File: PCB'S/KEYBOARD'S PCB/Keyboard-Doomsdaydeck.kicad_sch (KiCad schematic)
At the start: 2 parts, among them J5 Conn_01x04_Pin, U1 Raspberry_Pi_Pico2

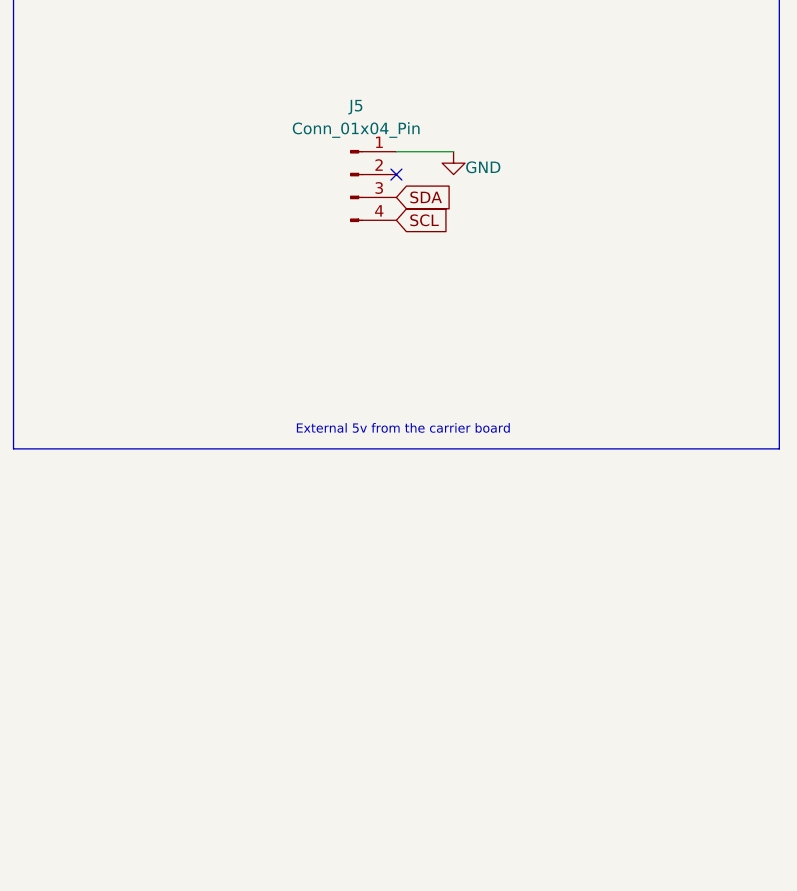
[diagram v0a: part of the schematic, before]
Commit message: ain
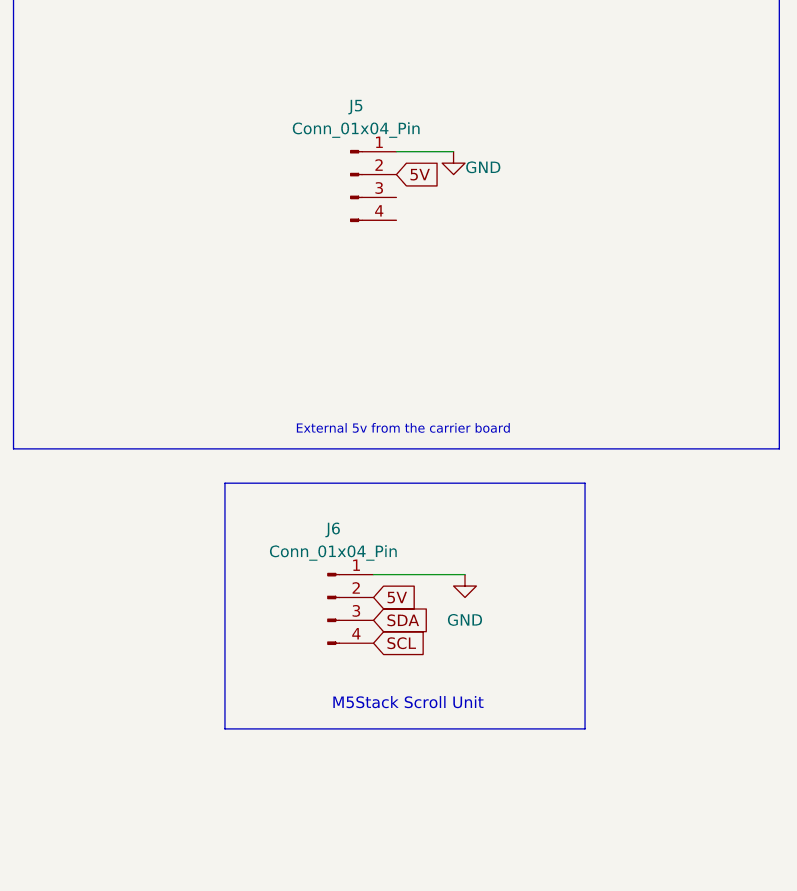
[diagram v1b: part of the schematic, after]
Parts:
- added J6: Conn_01x04_Pin, Connector:FanPinHeader_1x04_P2.54mm_Vertical, symbol Connector:Conn_01x04_Pin
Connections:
- net GND: now also J6.1 (Pin_1)
- net SCL: now also J6.4 (Pin_4); no longer J5.4 (Pin_4)
- net SDA: now also J6.3 (Pin_3); no longer J5.3 (Pin_3)
- net 5V: now reaches J5.2 (Pin_2)
- net 5V: now also J6.2 (Pin_2)
- no-connect marks 12 -> 11
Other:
- note added: "M5Stack Scroll Unit"
